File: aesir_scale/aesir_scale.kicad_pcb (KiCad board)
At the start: 2 copper layers, 60 x 50 mm, 56 parts, among them J1 jst xh 4, J2 jst gh, J3 jst xh 4, J4 jst_sh 6, J5 jst gh, J6 USB_C_Receptacle_USB2.0, U1 STM32U575CGTx, U2 NAU7802SGI, U3 AZ1117CH2-3.3TRG1, U4 TJA1051T, U5 USBLC6-2SC6, Y1 48MHz

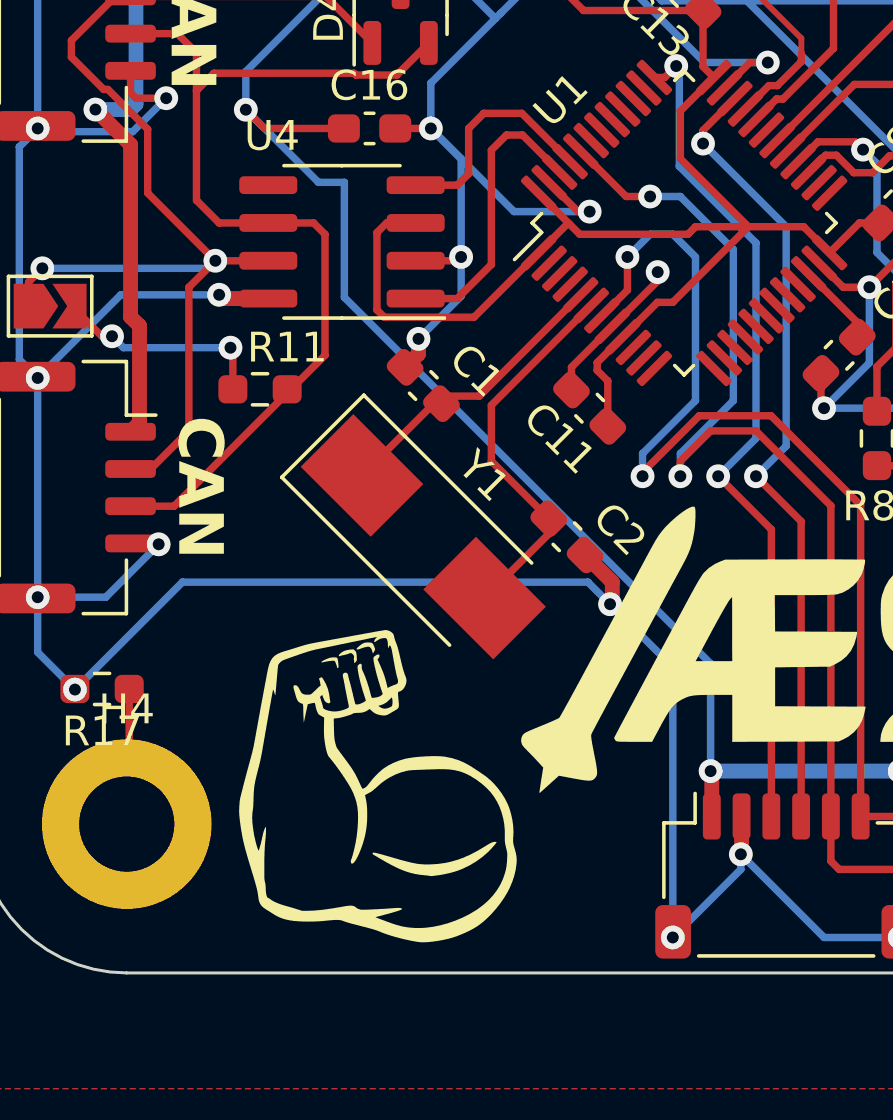
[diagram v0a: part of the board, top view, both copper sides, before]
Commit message: updated
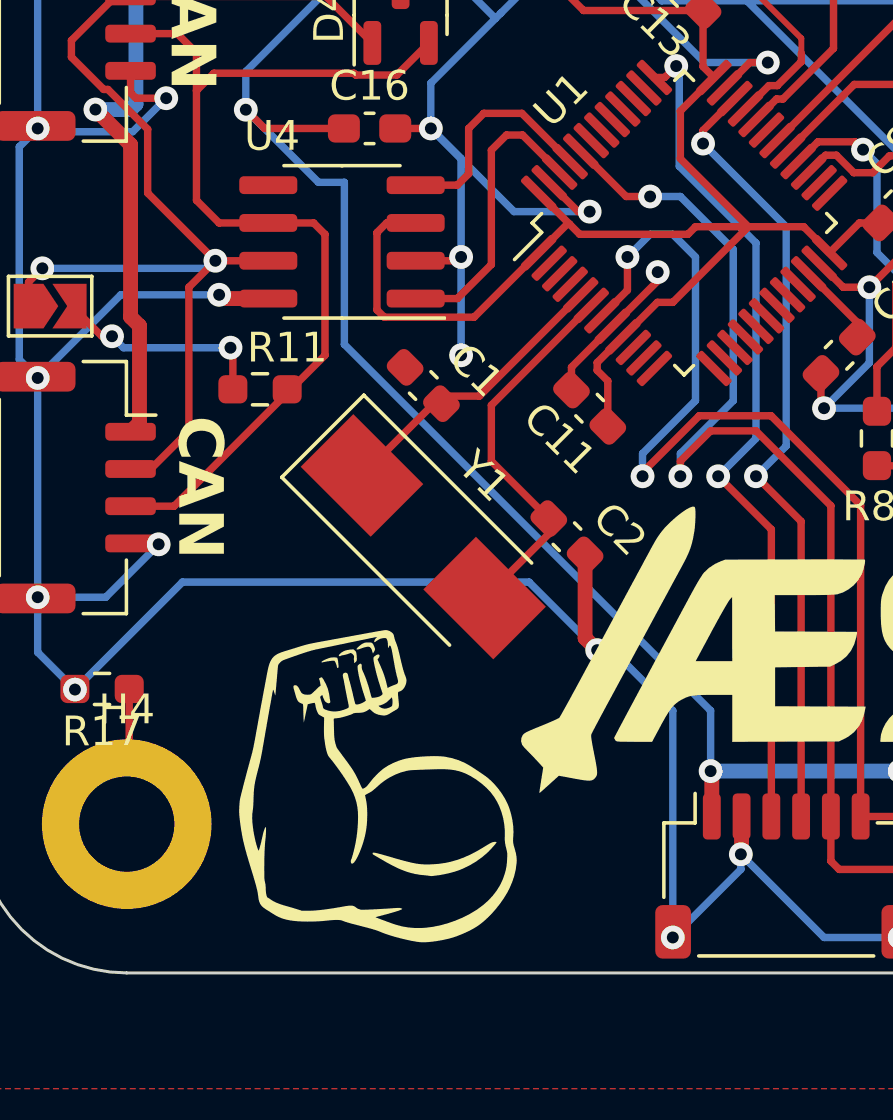
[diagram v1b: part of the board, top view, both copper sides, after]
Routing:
- net Earth: track 455.0 -> 454.3 mm
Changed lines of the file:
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@@
   (segment (start 92.954 114.818) (end 92.964 114.808) (width 0.5) (layer "F.Cu") (net 12))
   (segment (start 91.948 92.964) (end 93.853 91.059) (width 0.25) (layer "F.Cu") (net 12))
-  (segment (start 76.800625 95.207615) (end 76.800625 94.698203) (width 0.5) (layer "F.Cu") (net 12))
   (segment (start 67.48 75.57) (end 67.51 75.54) (width 0.25) (layer "F.Cu") (net 12))
-  (segment (start 76.35212 95.65612) (end 76.800625 95.207615) (width 0.5) (layer "F.Cu") (net 12))
   (segment (start 76.2 82.8825) (end 77.597348 81.485152) (width 0.25) (layer "F.Cu") (net 12))
   (segment (start 67.128 85.695) (end 67.128 86.432) (width 0.25) (layer "F.Cu") (net 12))
@@
   (segment (start 76.02 87.63) (end 77.216 87.63) (width 0.25) (layer "F.Cu") (net 12))
   (segment (start 81.28 80.898) (end 81.28 81.505484) (width 0.5) (layer "F.Cu") (net 12))
+  (segment (start 82.39788 104.74988) (end 82.804 105.156) (width 0.5) (layer "F.Cu") (net 12))
+  (segment (start 82.39788 101.95588) (end 82.39788 104.74988) (width 0.5) (layer "F.Cu") (net 12))
   (segment (start 82.904 73.1524) (end 82.4404 73.1524) (width 0.5) (layer "F.Cu") (net 12))
   (segment (start 102.235 88.0375) (end 102.235 85.6245) (width 0.5) (layer "F.Cu") (net 12))
@@
   (segment (start 87.95 79.005) (end 87.95 78.523874) (width 0.25) (layer "F.Cu") (net 12))
   (segment (start 89.304 73.1524) (end 89.7676 73.1524) (width 0.5) (layer "F.Cu") (net 12))
-  (segment (start 82.39788 101.95588) (end 83.312 102.87) (width 0.5) (layer "F.Cu") (net 12))
   (segment (start 87.077342 86.270678) (end 87.931668 85.416352) (width 0.25) (layer "F.Cu") (net 12))
   (segment (start 90.32212 95.85988) (end 90.32212 96.92612) (width 0.25) (layer "F.Cu") (net 12))
@@
   (segment (start 77.8775 81.205) (end 77.8775 80.924) (width 0.25) (layer "F.Cu") (net 12))
   (segment (start 67.128 86.432) (end 67.31 86.614) (width 0.25) (layer "F.Cu") (net 12))
-  (segment (start 83.312 102.87) (end 83.312 103.536378) (width 0.5) (layer "F.Cu") (net 12))
   (segment (start 90.32212 96.92612) (end 90.424 97.028) (width 0.25) (layer "F.Cu") (net 12))
   (segment (start 76.2 79.2465) (end 76.2 77.724) (width 0.5) (layer "F.Cu") (net 12))
-  (segment (start 83.312 103.536378) (end 83.236177 103.612201) (width 0.5) (layer "F.Cu") (net 12))
   (segment (start 87.654 110.744) (end 87.654 111.99) (width 0.5) (layer "F.Cu") (net 12))
   (segment (start 77.8775 80.924) (end 76.2 79.2465) (width 0.5) (layer "F.Cu") (net 12))
@@
   (via (at 91.948 92.964) (size 0.8) (drill 0.4) (layers "F.Cu" "B.Cu") (net 12))
   (via (at 70.104 93.218) (size 0.8) (drill 0.4) (layers "F.Cu" "B.Cu") (net 12))
-  (via (at 83.236177 103.612201) (size 0.8) (drill 0.4) (layers "F.Cu" "B.Cu") (net 12))
+  (via (at 82.804 105.156) (size 0.8) (drill 0.4) (layers "F.Cu" "B.Cu") (net 12))
   (via (at 98.298 86.36) (size 0.8) (drill 0.4) (layers "F.Cu" "B.Cu") (net 12))
   (via (at 78.232 91.948) (size 0.8) (drill 0.4) (layers "F.Cu" "B.Cu") (net 12))
@@
   (via (at 87.108063 77.681937) (size 0.8) (drill 0.4) (layers "F.Cu" "B.Cu") (free) (net 12))
   (via (at 85.344 114.808) (size 0.8) (drill 0.4) (layers "F.Cu" "B.Cu") (net 12))
-  (via (at 76.800625 94.698203) (size 0.8) (drill 0.4) (layers "F.Cu" "B.Cu") (net 12))
+  (via (at 78.232 95.25) (size 0.8) (drill 0.4) (layers "F.Cu" "B.Cu") (free) (net 12))
   (via (at 88.534648 85.416352) (size 0.8) (drill 0.4) (layers "F.Cu" "B.Cu") (net 12))
   (via (at 77.216 87.63) (size 0.8) (drill 0.4) (layers "F.Cu" "B.Cu") (net 12))
@@
   (segment (start 99.568 97.04) (end 99.58 97.028) (width 0.25) (layer "B.Cu") (net 12))
   (segment (start 81.548258 81.773742) (end 82.768339 81.773742) (width 0.25) (layer "B.Cu") (net 12))
-  (segment (start 85.344 114.808) (end 85.344 105.720024) (width 0.25) (layer "B.Cu") (net 12))
   (segment (start 63.39 88.248) (end 63.39 95.394) (width 0.25) (layer "B.Cu") (net 12))
   (segment (start 87.63 112.014) (end 90.424 114.808) (width 0.25) (layer "B.Cu") (net 12))
   (segment (start 64.008 105.228) (end 65.26 106.48) (width 0.25) (layer "B.Cu") (net 12))
-  (segment (start 65.26 106.48) (end 68.87 102.87) (width 0.25) (layer "B.Cu") (net 12))
   (segment (start 94.234 114.808) (end 92.964 114.808) (width 0.25) (layer "B.Cu") (net 12))
   (segment (start 110.928 97.028) (end 111.47 97.57) (width 0.25) (layer "B.Cu") (net 12))
@@
   (segment (start 99.568 97.536) (end 99.568 97.04) (width 0.25) (layer "B.Cu") (net 12))
   (segment (start 71.614 74.676) (end 64.008 82.282) (width 0.25) (layer "B.Cu") (net 12))
+  (segment (start 80.518 102.87) (end 82.804 105.156) (width 0.25) (layer "B.Cu") (net 12))
   (segment (start 91.948 92.964) (end 91.948 95.504) (width 0.25) (layer "B.Cu") (net 12))
-  (segment (start 85.344 105.720024) (end 83.236177 103.612201) (width 0.25) (layer "B.Cu") (net 12))
+  (segment (start 85.344 107.188) (end 83.312 105.156) (width 0.25) (layer "B.Cu") (net 12))
   (segment (start 79.566 83.756) (end 81.548258 81.773742) (width 0.25) (layer "B.Cu") (net 12))
   (segment (start 100.838 83.82) (end 98.298 86.36) (width 0.25) (layer "B.Cu") (net 12))
+  (segment (start 65.26 106.48) (end 68.87 102.87) (width 0.25) (layer "B.Cu") (net 12))
   (segment (start 68.374 74.676) (end 67.51 75.54) (width 0.25) (layer "B.Cu") (net 12))
   (segment (start 77.216 87.63) (end 80.01 90.424) (width 0.25) (layer "B.Cu") (net 12))
@@
   (segment (start 64.008 87.63) (end 64.118 87.74) (width 0.25) (layer "B.Cu") (net 12))
   (segment (start 102.108 83.82) (end 100.838 83.82) (width 0.25) (layer "B.Cu") (net 12))
+  (segment (start 68.87 102.87) (end 80.518 102.87) (width 0.25) (layer "B.Cu") (net 12))
   (segment (start 64.008 96.012) (end 64.008 103.378) (width 0.25) (layer "B.Cu") (net 12))
   (segment (start 106.75525 83.82) (end 102.108 83.82) (width 0.25) (layer "B.Cu") (net 12))
@@
   (segment (start 112.98 99.08) (end 111.47 97.57) (width 0.25) (layer "B.Cu") (net 12))
   (segment (start 70.104 93.218) (end 66.802 93.218) (width 0.25) (layer "B.Cu") (net 12))
+  (segment (start 78.232 91.948) (end 78.232 95.25) (width 0.25) (layer "B.Cu") (net 12))
   (segment (start 98.552 110.49) (end 94.234 114.808) (width 0.25) (layer "B.Cu") (net 12))
   (segment (start 90.424 97.028) (end 99.58 97.028) (width 0.25) (layer "B.Cu") (net 12))
-  (segment (start 78.232 93.266828) (end 76.800625 94.698203) (width 0.25) (layer "B.Cu") (net 12))
-  (segment (start 68.87 102.87) (end 82.493976 102.87) (width 0.25) (layer "B.Cu") (net 12))
   (segment (start 64.008 103.378) (end 64.008 105.228) (width 0.25) (layer "B.Cu") (net 12))
   (segment (start 78.430937 76.906937) (end 76.2 74.676) (width 0.25) (layer "B.Cu") (net 12))
@@
   (segment (start 76.2 74.676) (end 71.614 74.676) (width 0.25) (layer "B.Cu") (net 12))
   (segment (start 77.216 87.63) (end 78.232 88.646) (width 0.25) (layer "B.Cu") (net 12))
-  (segment (start 78.232 91.948) (end 78.232 93.266828) (width 0.25) (layer "B.Cu") (net 12))
+  (segment (start 83.312 105.156) (end 82.804 105.156) (width 0.25) (layer "B.Cu") (net 12))
   (segment (start 106.24725 74.676) (end 111.07325 79.502) (width 0.25) (layer "B.Cu") (net 12))
   (segment (start 77.597348 82.147348) (end 77.597348 80.757348) (width 0.25) (layer "B.Cu") (net 12))
   (segment (start 64.008 82.282) (end 64.008 87.63) (width 0.25) (layer "B.Cu") (net 12))
   (segment (start 98.552 110.49) (end 109.51 110.49) (width 0.25) (layer "B.Cu") (net 12))
-  (segment (start 82.493976 102.87) (end 83.236177 103.612201) (width 0.25) (layer "B.Cu") (net 12))
+  (segment (start 85.344 114.808) (end 85.344 107.188) (width 0.25) (layer "B.Cu") (net 12))
   (segment (start 77.216 87.63) (end 77.216 86.106) (width 0.25) (layer "B.Cu") (net 12))
   (segment (start 64.008 87.63) (end 63.39 88.248) (width 0.25) (layer "B.Cu") (net 12))
@@
   (segment (start 92.964 99.996) (end 93.98 98.98) (width 0.25) (layer "B.Cu") (net 13))
   (segment (start 99.858861 95.370002) (end 111.370002 95.370002) (width 0.25) (layer "B.Cu") (net 13))
-  (segment (start 86.614 109.22) (end 86.614 105.607594) (width 0.25) (layer "B.Cu") (net 13))
+  (segment (start 86.614 107.188) (end 74.31 94.884) (width 0.25) (layer "B.Cu") (net 13))
   (segment (start 80.08793 78.456937) (end 79.042867 79.502) (width 0.25) (layer "B.Cu") (net 13))
   (segment (start 82.945796 78.456937) (end 99.858861 95.370002) (width 0.25) (layer "B.Cu") (net 13))
-  (segment (start 74.31 93.303594) (end 74.31 89.44) (width 0.25) (layer "B.Cu") (net 13))
-  (segment (start 86.614 105.607594) (end 74.31 93.303594) (width 0.25) (layer "B.Cu") (net 13))
   (segment (start 84.972985 83.341992) (end 95.188008 83.341992) (width 0.25) (layer "B.Cu") (net 13))
   (segment (start 79.042867 79.502) (end 77.216 79.502) (width 0.25) (layer "B.Cu") (net 13))
   (segment (start 73.44 89.44) (end 71 87) (width 0.25) (layer "B.Cu") (net 13))
+  (segment (start 74.31 89.44) (end 73.44 89.44) (width 0.25) (layer "B.Cu") (net 13))
   (segment (start 80.08793 78.456937) (end 84.972985 83.341992) (width 0.25) (layer "B.Cu") (net 13))
   (segment (start 92.964 109.22) (end 92.964 105.656) (width 0.25) (layer "B.Cu") (net 13))
@@
   (segment (start 80.08793 78.456937) (end 82.945796 78.456937) (width 0.25) (layer "B.Cu") (net 13))
   (segment (start 71 85.718) (end 71 87) (width 0.25) (layer "B.Cu") (net 13))
-  (segment (start 74.31 89.44) (end 73.44 89.44) (width 0.25) (layer "B.Cu") (net 13))
+  (segment (start 86.614 109.22) (end 86.614 107.188) (width 0.25) (layer "B.Cu") (net 13))
+  (segment (start 74.31 94.884) (end 74.31 89.44) (width 0.25) (layer "B.Cu") (net 13))
   (segment (start 75.25 84.7575) (end 73.6875 83.195) (width 0.25) (layer "F.Cu") (net 32))
   (segment (start 63.701 93.599) (end 63.701 92.793) (width 0.25) (layer "F.Cu") (net 32))

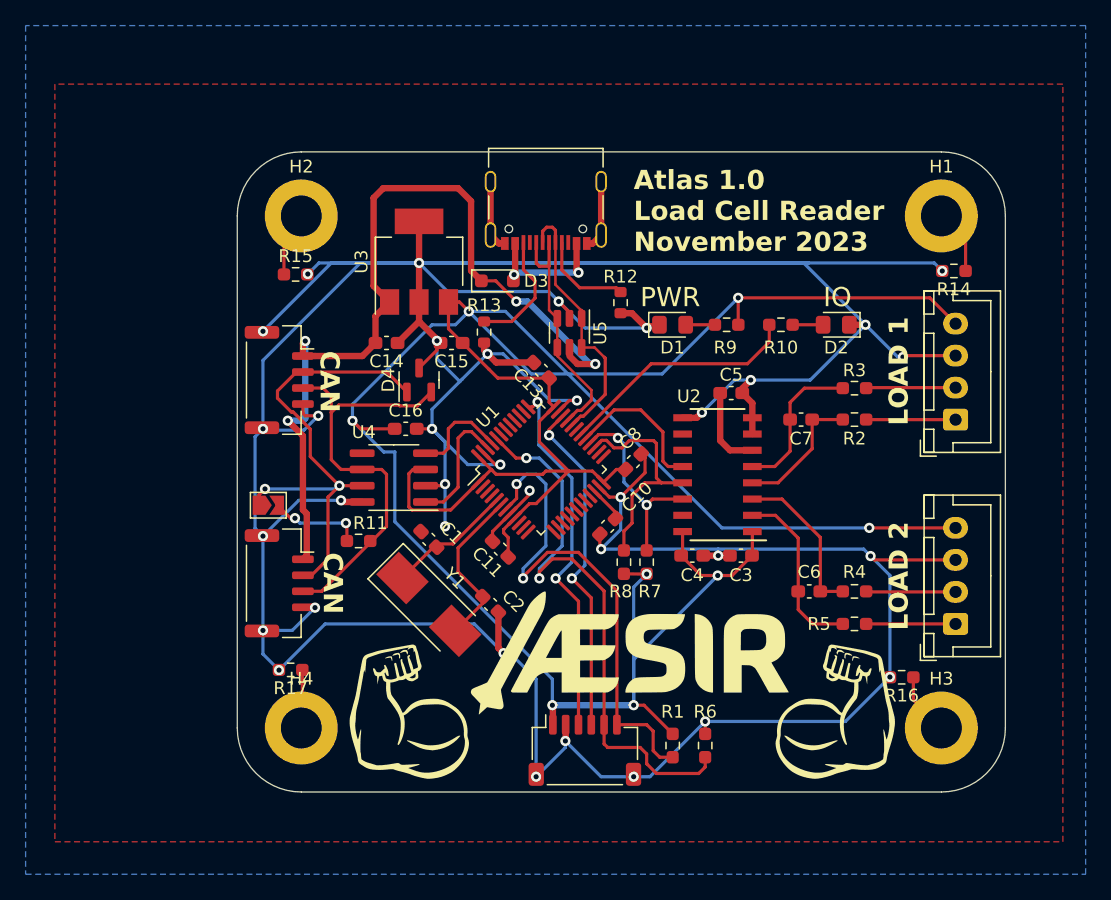
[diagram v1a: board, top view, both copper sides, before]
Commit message: updated
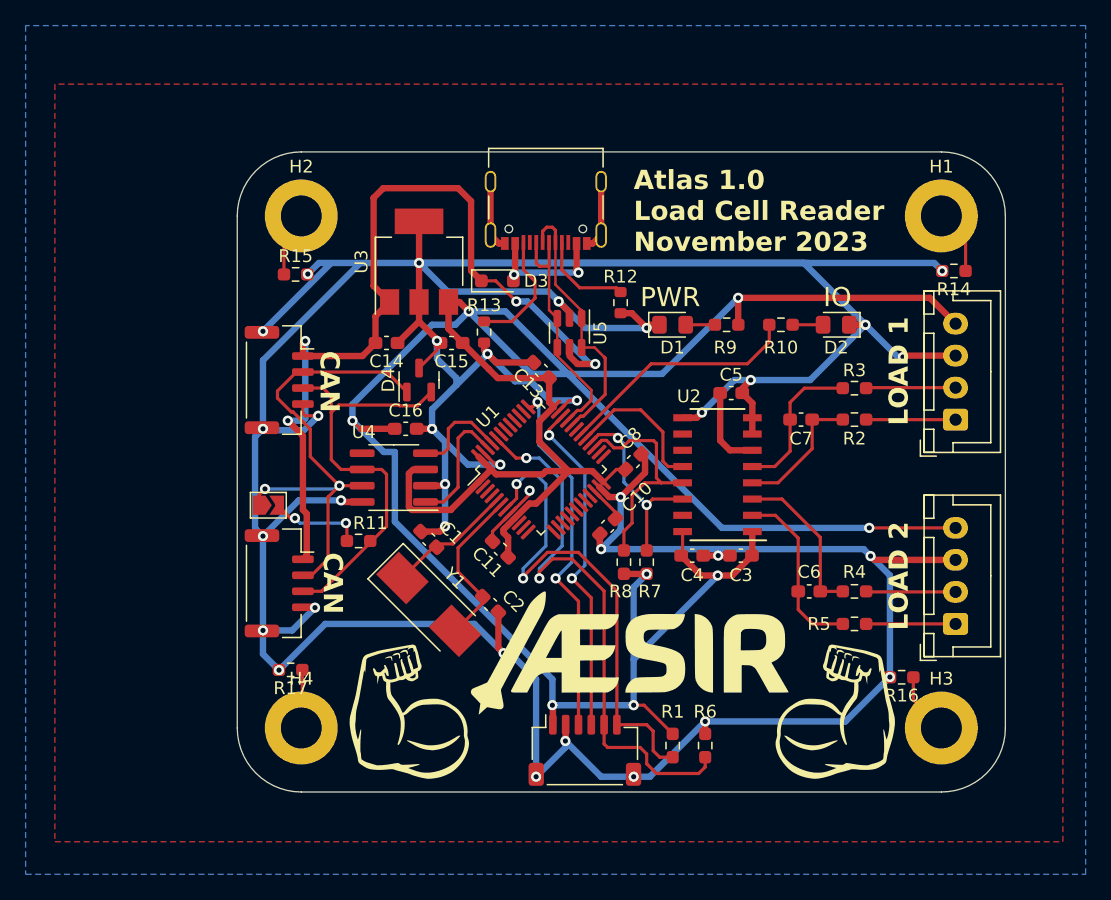
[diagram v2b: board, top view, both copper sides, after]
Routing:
- net Earth: track 454.3 -> 456.5 mm
